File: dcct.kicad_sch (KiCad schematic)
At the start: 53 parts, among them U32 LTC6655BHLS8-5, U33 AD8429BRZ, U34 AD8675ARZ, U35 LT6202CS5, U36 LTC6363xMS8, U37 LTC2376CDE-20-PBF

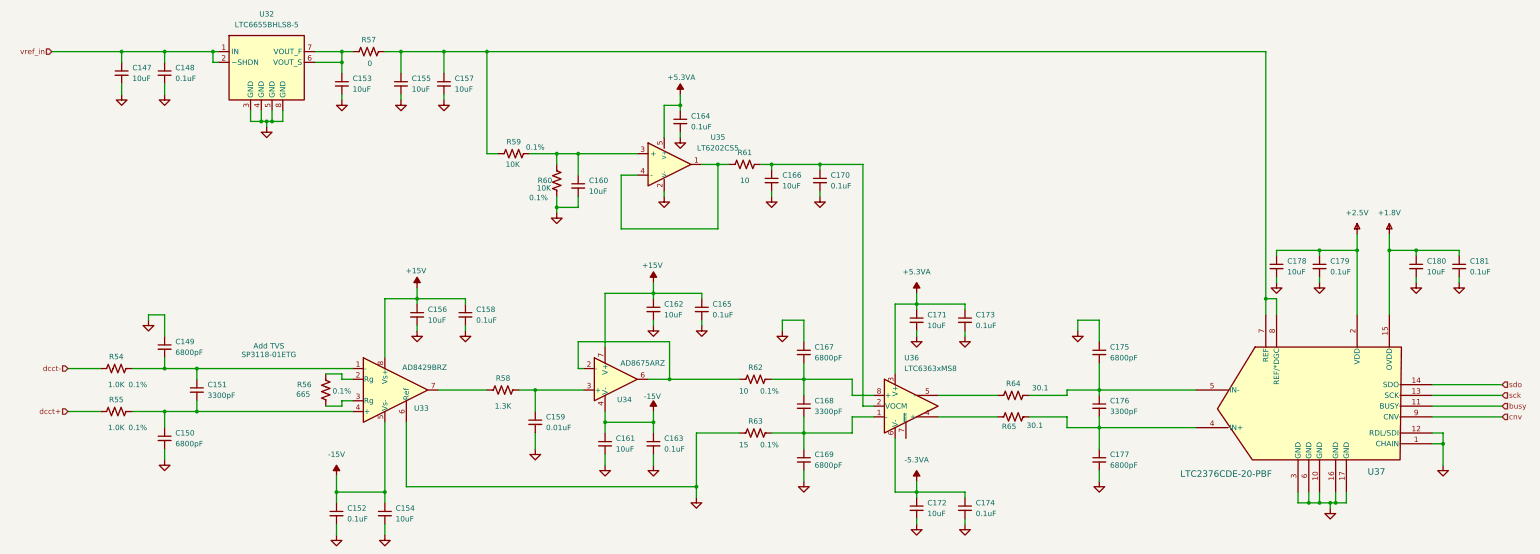
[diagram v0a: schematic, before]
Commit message: finish rough placement
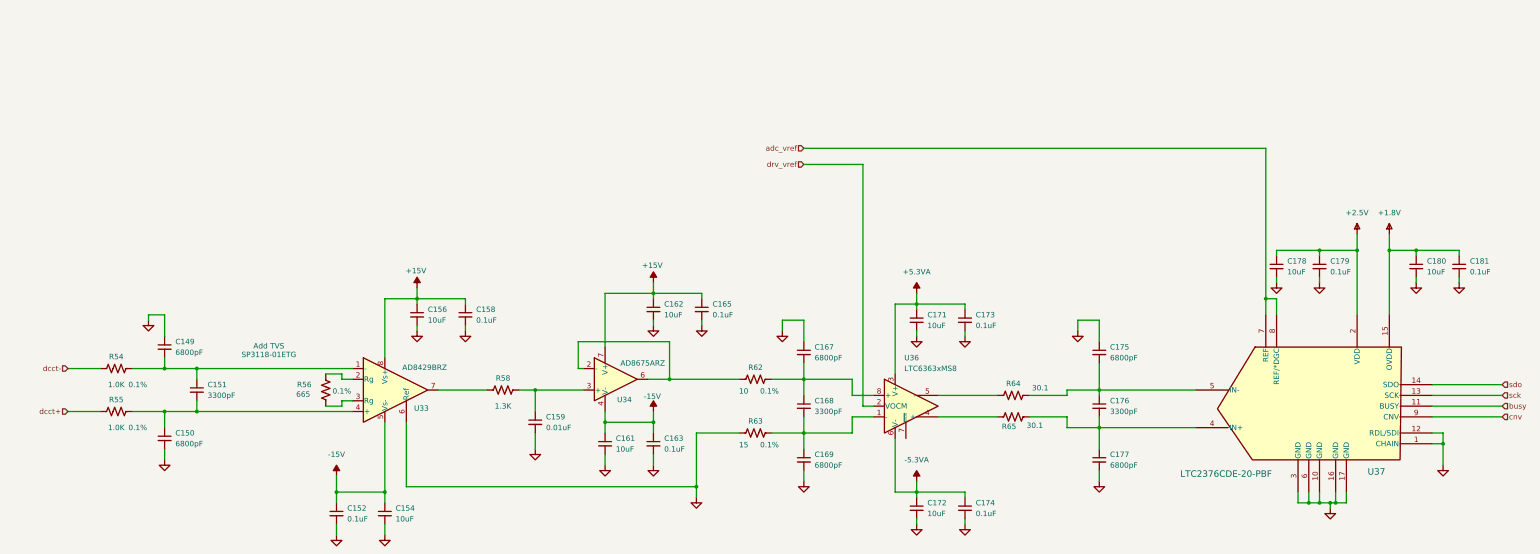
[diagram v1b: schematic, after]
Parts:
- removed C147, C153, C155, C157, C160, C166: 10uF, Capacitor_SMD:C_0603_1608Metric, symbol Device:C_Small
- removed C148, C164, C170: 0.1uF, Capacitor_SMD:C_0402_1005Metric, symbol Device:C_Small
- removed R57: 0, Resistor_SMD:R_0402_1005Metric, symbol Device:R_US
- removed R59, R60: 10K, Resistor_SMD:R_0402_1005Metric, symbol Device:R_US
- removed R61: 10, Resistor_SMD:R_0402_1005Metric, symbol Device:R_US
- removed U32: LTC6655BHLS8-5, myparts:LTC6655, symbol PSC:LTC6655BHLS8-5
- removed U35: LT6202CS5, myparts:LT6202CS5, symbol PSC:LT6202CS5
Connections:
- net drv_vref: now reaches U36.2 (VOCM)
- net adc_vref: now reaches U37.7 (REF), U37.8 (REF/*DGC)
